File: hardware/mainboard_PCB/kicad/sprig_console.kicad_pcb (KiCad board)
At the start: 2 copper layers, 139.7 x 64.8 mm, 42 parts, among them J1 1020_battery_holder, J2 Conn_PinHeader_2x03_P2.54mm_V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, SW1 W, SW2 A, SW3 S, SW4 D, SW5 I, SW6 J, SW7 K, SW8 L, SW9 Slideswitch, U1 Adafruit_TFT_ST7735, U2 MAX98357AETE+, U5 Pico

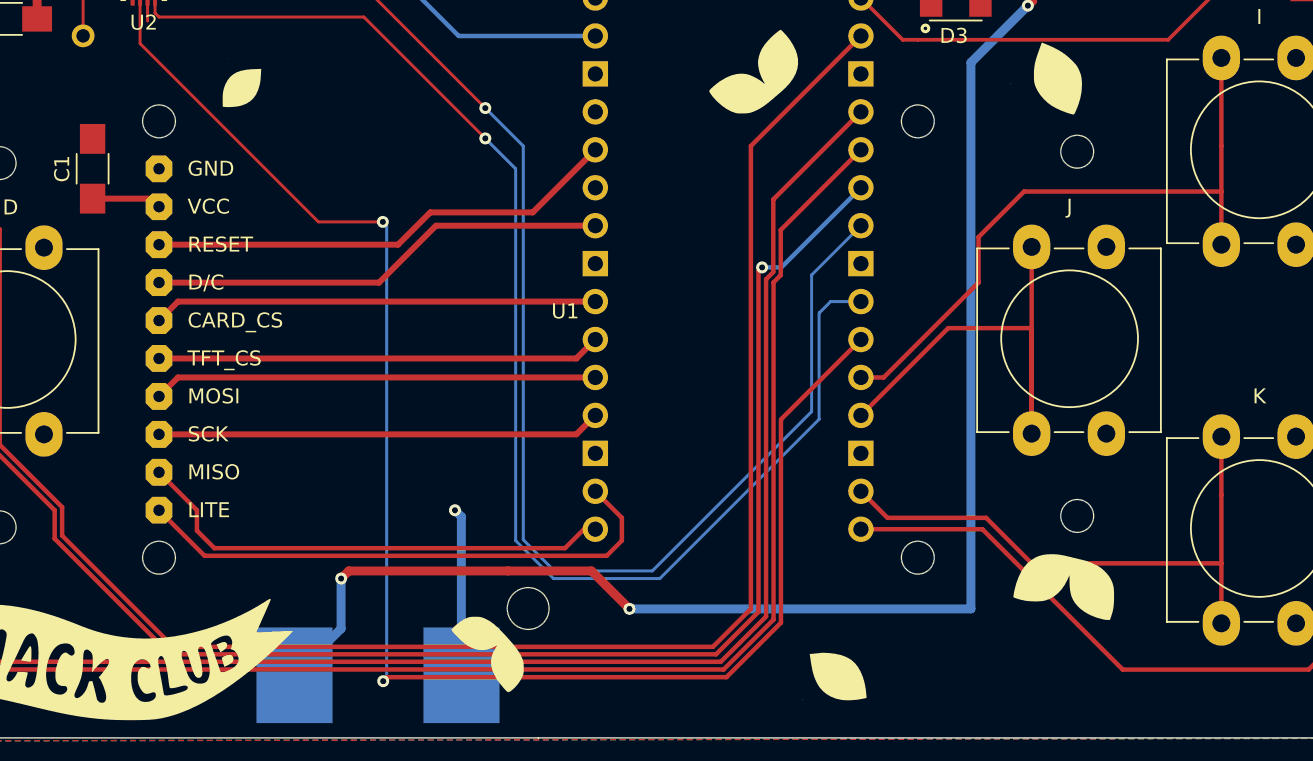
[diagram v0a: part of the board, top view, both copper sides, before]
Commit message: new board for new screen (#2430)
* new board design w/ cheaper screens

* new board design w/ cheaper screens

* add nora as co author

Co-authored-by: Nora <nora@hackclub.com>

* try again

wahoo



Co-authored-by: Nora <nora@hackclub.com>

* Update fp-lib-table


Co-authored-by: 24c02 <163450896+24c02@users.noreply.github.com>

---------

Co-authored-by: Nora <nora@hackclub.com>
Co-authored-by: 24c02 <163450896+24c02@users.noreply.github.com>
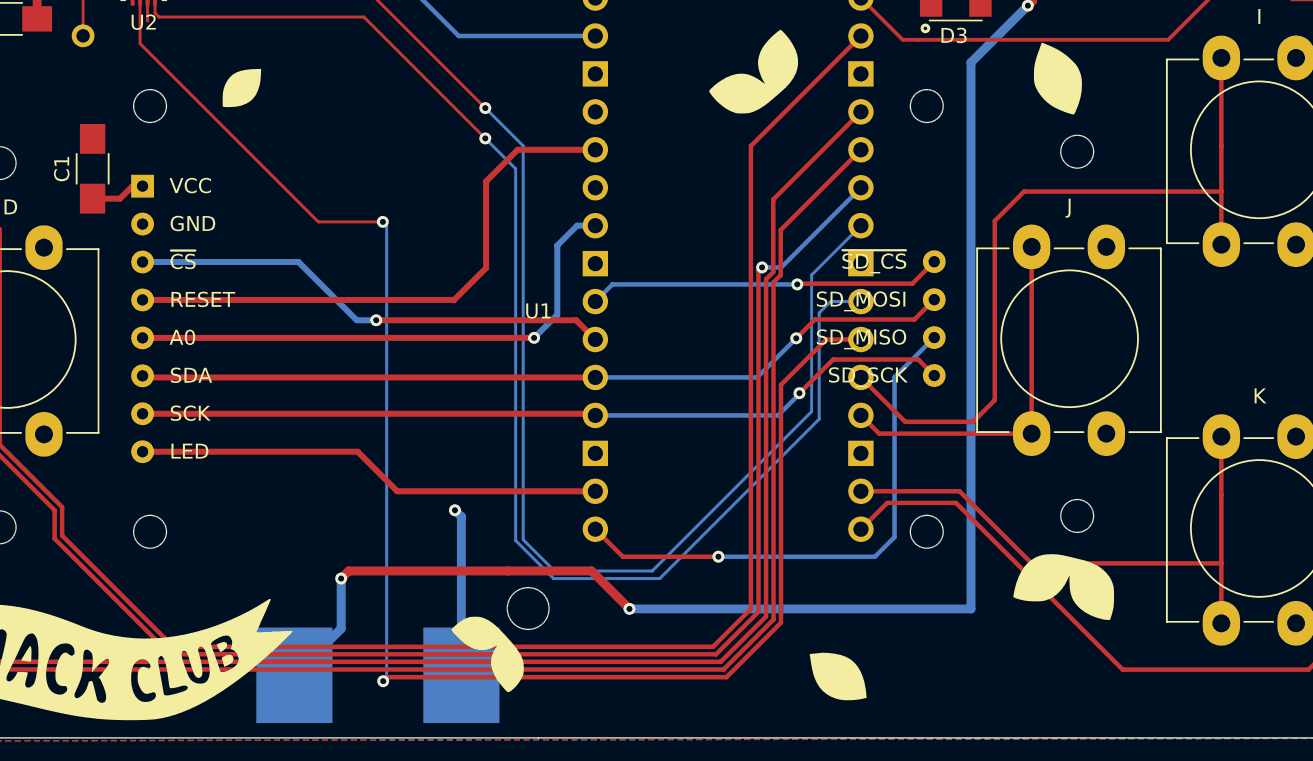
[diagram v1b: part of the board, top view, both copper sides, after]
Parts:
- U1: value Adafruit_TFT_ST7735 -> ~; footprint fab:TFT_ST7735 -> sprig:TFT_MSP1803
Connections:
- U1 pad 1: LITE -> +3V3
- U1 pad 10: GND -> MOSI
- U1 pad 2: MISO -> GND
- U1 pad 3: SCK -> TFT_CS
- U1 pad 4: MOSI -> RESET
- U1 pad 5: TFT_CS -> D/C
- U1 pad 6: CARD_CS -> MOSI
- U1 pad 7: D/C -> SCK
- U1 pad 8: RESET -> LITE
- U1 pad 9: +3V3 -> CARD_CS
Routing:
- net MOSI: track 29.7 -> 55.6 mm, vias 0 -> 1
- net SCK: track 29.7 -> 55.3 mm, vias 0 -> 1
- net BTN_J: track 33.4 -> 24.4 mm
- net BTN_I: track 43.6 -> 51.9 mm
- net RESET: track 32.3 -> 38.6 mm
- net D/C: track 30.8 -> 36.7 mm, vias 0 -> 1
- net CARD_CS: track 29.7 -> 23.8 mm, vias 0 -> 1
- net LITE: track 36.7 -> 31.4 mm
- net MISO: track 32.6 -> 35.8 mm, vias 0 -> 1
- net TFT_CS: track 29.7 -> 32.5 mm, vias 0 -> 1
- net BTN_L: track 65.0 -> 66.4 mm
- net LRCLK: track 104.8 -> 106.1 mm
- net +3V3: track 16.9 -> 15.9 mm
